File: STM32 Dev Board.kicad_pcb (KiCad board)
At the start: 2 copper layers, 41.1 x 50 mm, 33 parts, among them J5 2 Pin JST, J6 USB_B_Micro, Q1 PMOS, U1 FT230XS, U2 STM32F070F6Px, U3 MCP1824S, U4 MCP73113

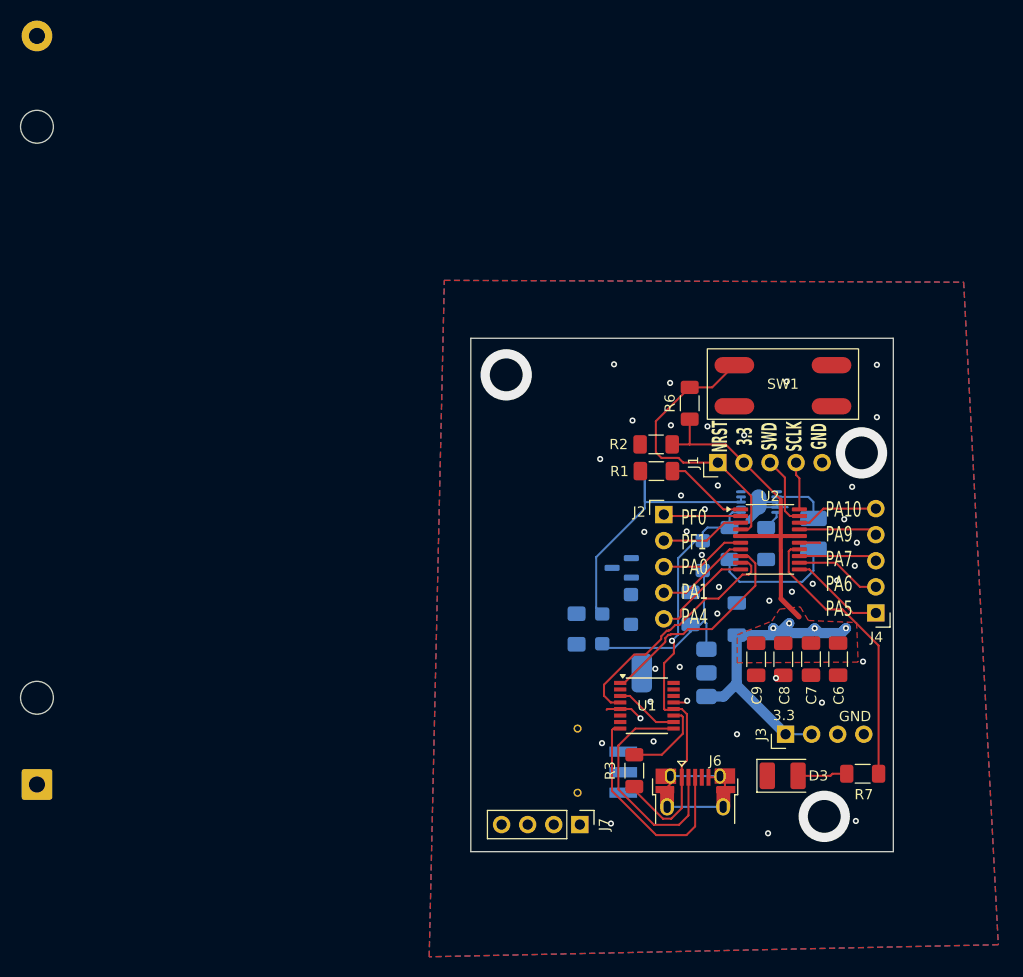
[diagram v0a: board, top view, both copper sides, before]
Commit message: generated drill and gerber files, updeted a few datasheets
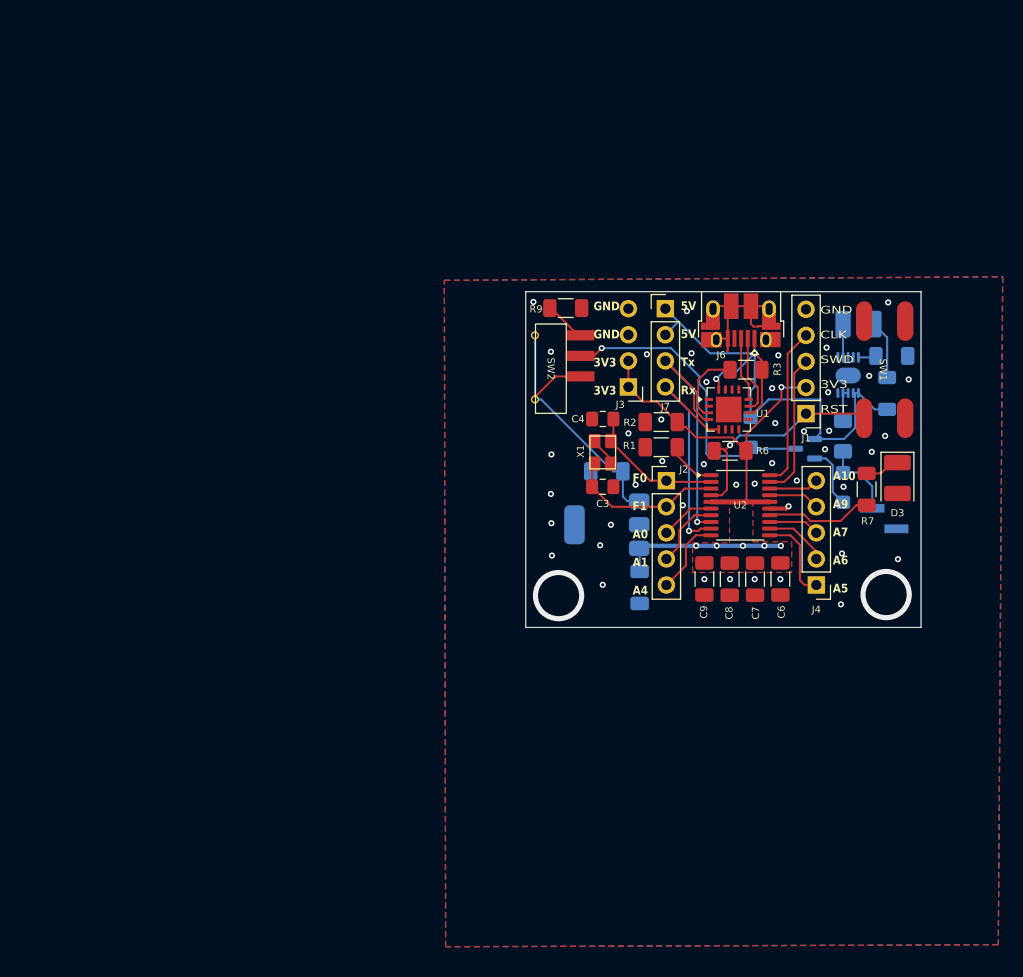
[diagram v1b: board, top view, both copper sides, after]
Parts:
- removed the D4 at (130.7, 97.0)
- removed the D4 at (127.8, 98.8)
- added C3: 7pF, Capacitor_SMD:C_0805_2012Metric_Pad1.18x1.45mm_HandSolder, F.Cu at (127.9, 85.0)
- added C4: 7pF, Capacitor_SMD:C_0805_2012Metric_Pad1.18x1.45mm_HandSolder, F.Cu at (127.9, 78.4)
- added D4: D_Schottky, Diode_SMD:D_SMF, B.Cu at (151.3, 85.1)
- added R9: 10k, Resistor_SMD:R_1206_3216Metric_Pad1.30x1.75mm_HandSolder, F.Cu at (124.3, 67.6)
- added X1: ~, MyLib:Xtal, F.Cu at (127.1, 82.8)
- J5: footprint Battery:BatteryHolder_MPD_BK-18650-PC2 -> Connector_PinHeader_2.00mm:PinHeader_1x02_P2.00mm_Vertical_SMD_Pin1Right
- SW2: moved to F.Cu
- U1: value FT230XS -> MCP2221AxML; footprint Package_SO:SSOP-16_3.9x4.9mm_P0.635mm -> Package_DFN_QFN:QFN-16-1EP_4x4mm_P0.65mm_EP2.5x2.5mm
- moved J5 86.5 mm to (155.3, 88.1), turned to 180 degrees
- moved J7 50.9 mm to (134.0, 67.7), turned to 0 degrees
- moved J6 46.5 mm to (141.3, 68.8), turned to 180 degrees
- moved SW2 40.8 mm to (125.3, 72.2), turned to -90 degrees
- moved R3 40.5 mm to (141.8, 73.6), turned to 180 degrees
- moved J3 37.1 mm to (130.4, 75.3), turned to 180 degrees
- moved R8 32.0 mm to (151.3, 80.1)
- moved D3 31.1 mm to (156.6, 84.2), turned to -90 degrees
- moved U1 29.9 mm to (140.2, 77.5)
- moved R7 27.7 mm to (153.6, 85.2), turned to -90 degrees
- moved R5 22.0 mm to (156.1, 72.3), turned to 0 degrees
- moved Q1 21.3 mm to (147.6, 81.3)
- moved R4 21.2 mm to (155.6, 75.9), turned to -90 degrees
- moved D1 20.9 mm to (152.8, 69.2), turned to 0 degrees
- moved U4 17.0 mm to (152.8, 72.6), turned to 180 degrees
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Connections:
- J7 pad 3: UART_Rx -> UART_Tx
- J7 pad 4: UART_Tx -> UART_Rx
- R3 pad 1: Net-(U1-~{RESET}) -> VUSB
- R3 pad 2: VUSB -> Net-(U1-~{RST})
- SW2 pad 1: GND -> Net-(R9-Pad1)
- U1 pad 1: UART_Tx -> unconnected-(U1-GP0-Pad1)
- U1 pad 10: Net-(U1-3V3OUT) -> VUSB
- U1 pad 11: Net-(U1-~{RESET}) -> Net-(J6-D-)
- U1 pad 12: VUSB -> Net-(J6-D+)
- U1 pad 16: unconnected-(U1-CBUS3-Pad16) -> VUSB
- U1 pad 3: Net-(U1-3V3OUT) -> Net-(U1-~{RST})
- U1 pad 4: UART_Rx -> UART_Tx
- U1 pad 5: GND -> UART_Rx
- U1 pad 8: Net-(J6-D+) -> unconnected-(U1-SDA-Pad8)
- U1 pad 9: Net-(J6-D-) -> unconnected-(U1-SCL-Pad9)
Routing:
- net Net-(SW2-C): track 0.00 -> 27.4 mm
- net /PSU/BAT+: track 29.9 -> 3.20 mm
- net Net-(U2-PB1): track 27.3 -> 10.4 mm
- net Net-(J6-D+): track 21.8 -> 6.24 mm
- net 3.3V: track 68.4 -> 53.5 mm, vias 4 -> 6
- net Net-(J6-D-): track 22.7 -> 7.69 mm
- net VUSB: track 43.5 -> 56.6 mm, vias 1 -> 2
- net /MCU/SWCLK: track 4.68 -> 15.7 mm
- net Net-(D2-K): track 19.4 -> 30.2 mm, vias 0 -> 1
- net GND: track 28.9 -> 20.0 mm, vias 42 -> 47
- net Net-(U1-~{RESET}): track 8.17 -> 0.00 mm
- net Net-(D4-A): track 0.00 -> 7.62 mm
- net Net-(U1-~{RST}): track 0.00 -> 7.44 mm
- net Net-(U2-PF1): track 8.20 -> 15.5 mm
- net /MCU/SWD: track 6.92 -> 14.0 mm
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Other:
- board size 41.1 x 50 mm -> 38.5 x 32.7 mm
- board text added: "5V 5V Tx Rx"
- board text added: "A10 A9 A7 A6 A5"
- board text added: "F0 F1 A0 A1 A4"
- board text added: "GND CLK SWD 3V3 RST"
- board text added: "GND GND 3V3 3V3"
- board text added: "Tyler Hickling STM32F070 Prototype Board V2.0 JUN/2026"
- board text removed: "3.3"
- board text removed: "GND"
- board text removed: "NRST 3.3 SWD SCLK GND"
- board text removed: "PA10 PA9 PA7 PA6 PA5"
- board text removed: "PF0 PF1 PA0 PA1 PA4"
